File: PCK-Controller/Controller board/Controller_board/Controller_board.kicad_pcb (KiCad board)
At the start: 2 copper layers, 2 parts, among them SW1 SW_Push, U1 EC10E1260507

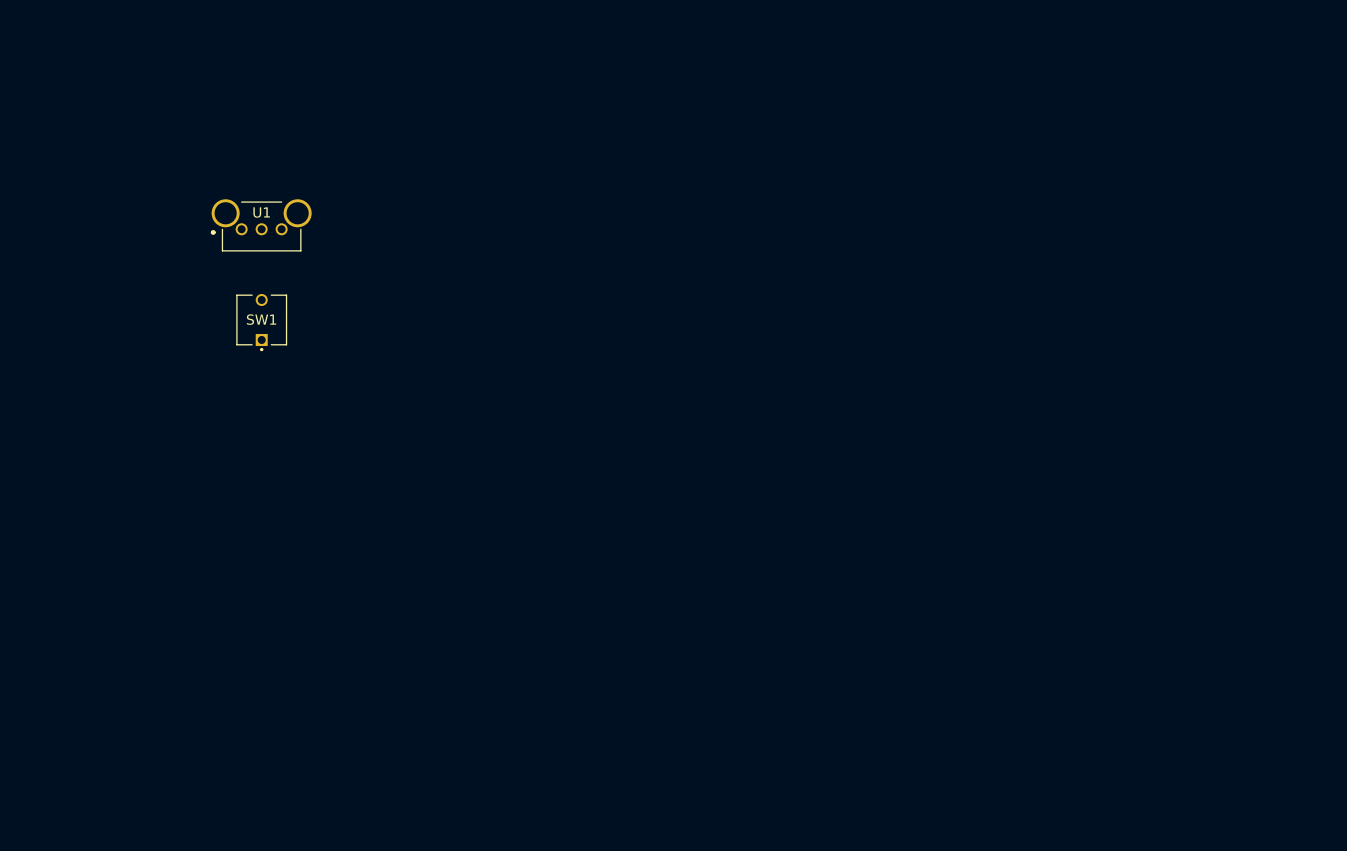
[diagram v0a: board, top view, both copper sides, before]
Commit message: Dimensions draft
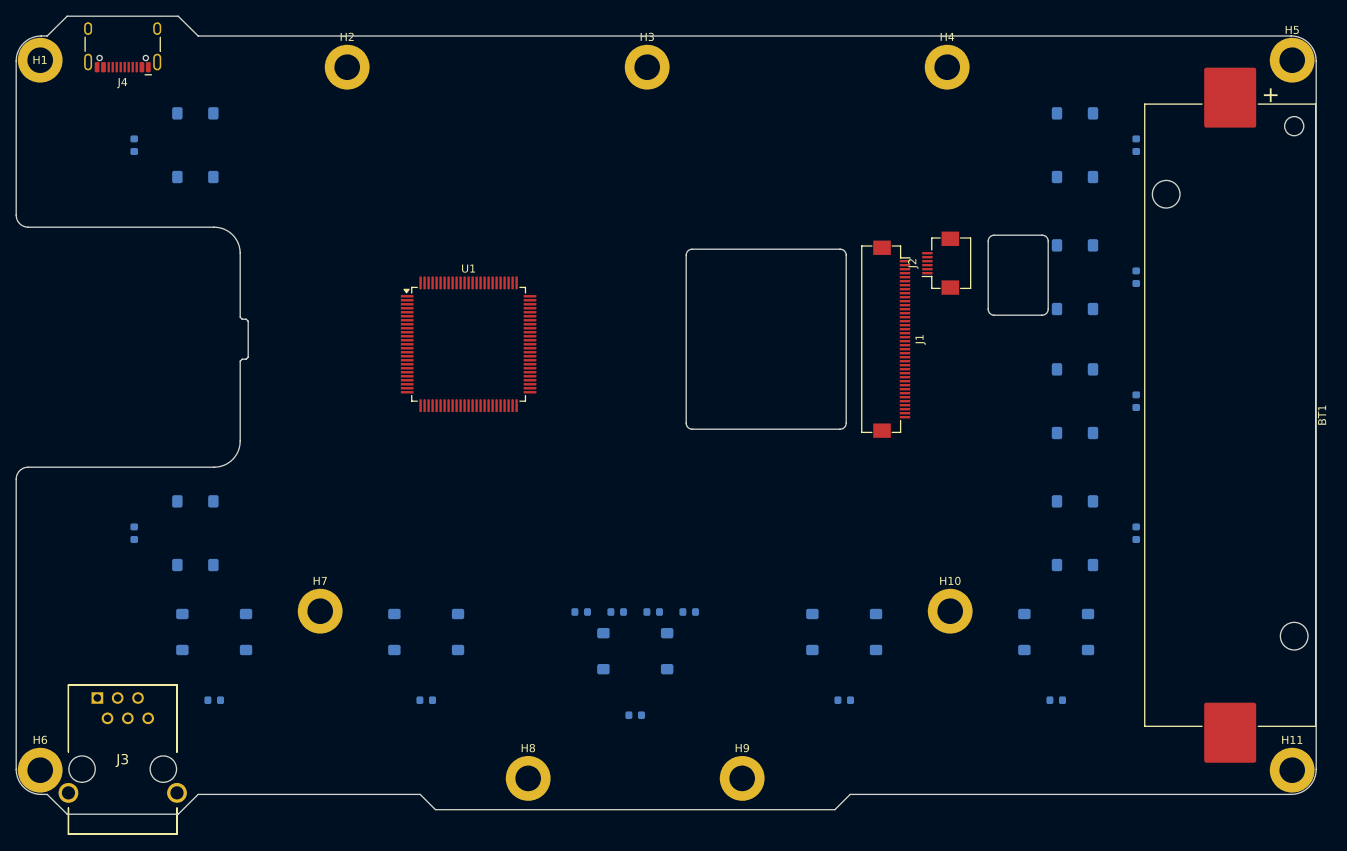
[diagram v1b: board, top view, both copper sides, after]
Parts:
- added BT1: Battery_Cell, Battery:BatteryHolder_Keystone_1042_1x18650, F.Cu at (220.5, 100.0)
- added D1: LED, LED_SMD:LED_0603_1608Metric, B.Cu at (152.9, 124.6)
- added D10: LED, LED_SMD:LED_0603_1608Metric, B.Cu at (172.2, 135.6)
- added D11: LED, LED_SMD:LED_0603_1608Metric, B.Cu at (146.1, 137.5)
- added D12: LED, LED_SMD:LED_0603_1608Metric, B.Cu at (120.0, 135.6)
- added D13: LED, LED_SMD:LED_0603_1608Metric, B.Cu at (93.5, 135.6)
- added D14: LED, LED_SMD:LED_0603_1608Metric, B.Cu at (83.5, 114.8)
- added D15: LED, LED_SMD:LED_0603_1608Metric, B.Cu at (83.5, 66.2)
- added D2: LED, LED_SMD:LED_0603_1608Metric, B.Cu at (148.4, 124.6)
- added D3: LED, LED_SMD:LED_0603_1608Metric, B.Cu at (143.9, 124.6)
- added D4: LED, LED_SMD:LED_0603_1608Metric, B.Cu at (139.4, 124.6)
- added D5: LED, LED_SMD:LED_0603_1608Metric, B.Cu at (208.8, 66.2)
- added D6: LED, LED_SMD:LED_0603_1608Metric, B.Cu at (208.8, 82.8)
- added D7: LED, LED_SMD:LED_0603_1608Metric, B.Cu at (208.8, 98.2)
- added D8: LED, LED_SMD:LED_0603_1608Metric, B.Cu at (208.8, 114.8)
- added D9: LED, LED_SMD:LED_0603_1608Metric, B.Cu at (198.8, 135.6)
- added H1: MountingHole_Pad, MountingHole:MountingHole_3.2mm_M3_DIN965_Pad, F.Cu at (71.8, 55.6)
- added H10: MountingHole_Pad, MountingHole:MountingHole_3.2mm_M3_DIN965_Pad, F.Cu at (185.5, 124.5)
- added H11: MountingHole_Pad, MountingHole:MountingHole_3.2mm_M3_DIN965_Pad, F.Cu at (228.2, 144.4)
- added H2: MountingHole_Pad, MountingHole:MountingHole_3.2mm_M3_DIN965_Pad, F.Cu at (110.1, 56.5)
- added H3: MountingHole_Pad, MountingHole:MountingHole_3.2mm_M3_DIN965_Pad, F.Cu at (147.6, 56.5)
- added H4: MountingHole_Pad, MountingHole:MountingHole_3.2mm_M3_DIN965_Pad, F.Cu at (185.1, 56.5)
- added H5: MountingHole_Pad, MountingHole:MountingHole_3.2mm_M3_DIN965_Pad, F.Cu at (228.2, 55.6)
- added H6: MountingHole_Pad, MountingHole:MountingHole_3.2mm_M3_DIN965_Pad, F.Cu at (71.8, 144.4)
- added H7: MountingHole_Pad, MountingHole:MountingHole_3.2mm_M3_DIN965_Pad, F.Cu at (106.8, 124.5)
- added H8: MountingHole_Pad, MountingHole:MountingHole_3.2mm_M3_DIN965_Pad, F.Cu at (132.8, 145.4)
- added H9: MountingHole_Pad, MountingHole:MountingHole_3.2mm_M3_DIN965_Pad, F.Cu at (159.5, 145.4)
- added J1: Conn_01x40, FPC_P0.50mm_Horizontal_40P:FPC_P0.50mm_Horizontal_40P, F.Cu at (178.0, 90.5)
- added J2: Conn_01x06, FPC_P0.50mm_Horizontal_40P:Hirose_FH12-6S-0.5SH_1x06-1MP_P0.50mm_Horizontal, F.Cu at (184.5, 81.0)
- added J3: RJE05-166-1310, SamacSys_Parts.pretty:RJE051661310, F.Cu at (78.9, 135.3)
- added J4: USB_C_Receptacle_USB2.0_14P, Connector_USB:USB_C_Receptacle_HCTL_HC-TYPE-C-16P-01A, F.Cu at (82.1, 52.8)
- added SW10: SW_Push, Button_Switch_SMD:SW_SPST_PTS645Sx43SMTR92, B.Cu at (91.2, 114.8)
- added SW11: SW_Push, Button_Switch_SMD:SW_SPST_PTS645Sx43SMTR92, B.Cu at (91.2, 66.2)
- added SW2: SW_Push, Button_Switch_SMD:SW_SPST_PTS645Sx43SMTR92, B.Cu at (201.1, 66.2)
- added SW3: SW_Push, Button_Switch_SMD:SW_SPST_PTS645Sx43SMTR92, B.Cu at (201.1, 82.8)
- added SW4: SW_Push, Button_Switch_SMD:SW_SPST_PTS645Sx43SMTR92, B.Cu at (201.1, 98.2)
- added SW5: SW_Push, Button_Switch_SMD:SW_SPST_PTS645Sx43SMTR92, B.Cu at (201.1, 114.8)
- added SW6: SW_Push, Button_Switch_SMD:SW_SPST_PTS645Sx43SMTR92, B.Cu at (198.8, 127.1)
- added SW7: SW_Push, Button_Switch_SMD:SW_SPST_PTS645Sx43SMTR92, B.Cu at (172.2, 127.1)
- added SW8: SW_Push, Button_Switch_SMD:SW_SPST_PTS645Sx43SMTR92, B.Cu at (120.0, 127.1)
- added SW9: SW_Push, Button_Switch_SMD:SW_SPST_PTS645Sx43SMTR92, B.Cu at (93.5, 127.1)
- SW1: footprint SamacSys_Parts.pretty:EVQP0E07K -> Button_Switch_SMD:SW_SPST_PTS645Sx43SMTR92; moved to B.Cu
- U1: value EC10E1260507 -> STM32U575VITx; footprint SamacSys_Parts.pretty:EC10E1260507 -> Package_QFP:LQFP-100_14x14mm_P0.5mm
- moved SW1 60.8 mm to (146.1, 129.5), turned to 0 degrees
- moved U1 31.8 mm to (125.3, 91.1)
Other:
- board outline added: 162.5 x 99.8 mm
